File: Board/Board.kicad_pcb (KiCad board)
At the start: 2 copper layers, 71.1 x 58.4 mm, 16 parts, among them J1 Bluetooth, J2 Conn_01x04_Female, J4 Conn_01x03_Female, J5 Conn_01x04_Female, J6 Voltage In 1, J7 Voltage In 2, J8 TrnasistorNPN

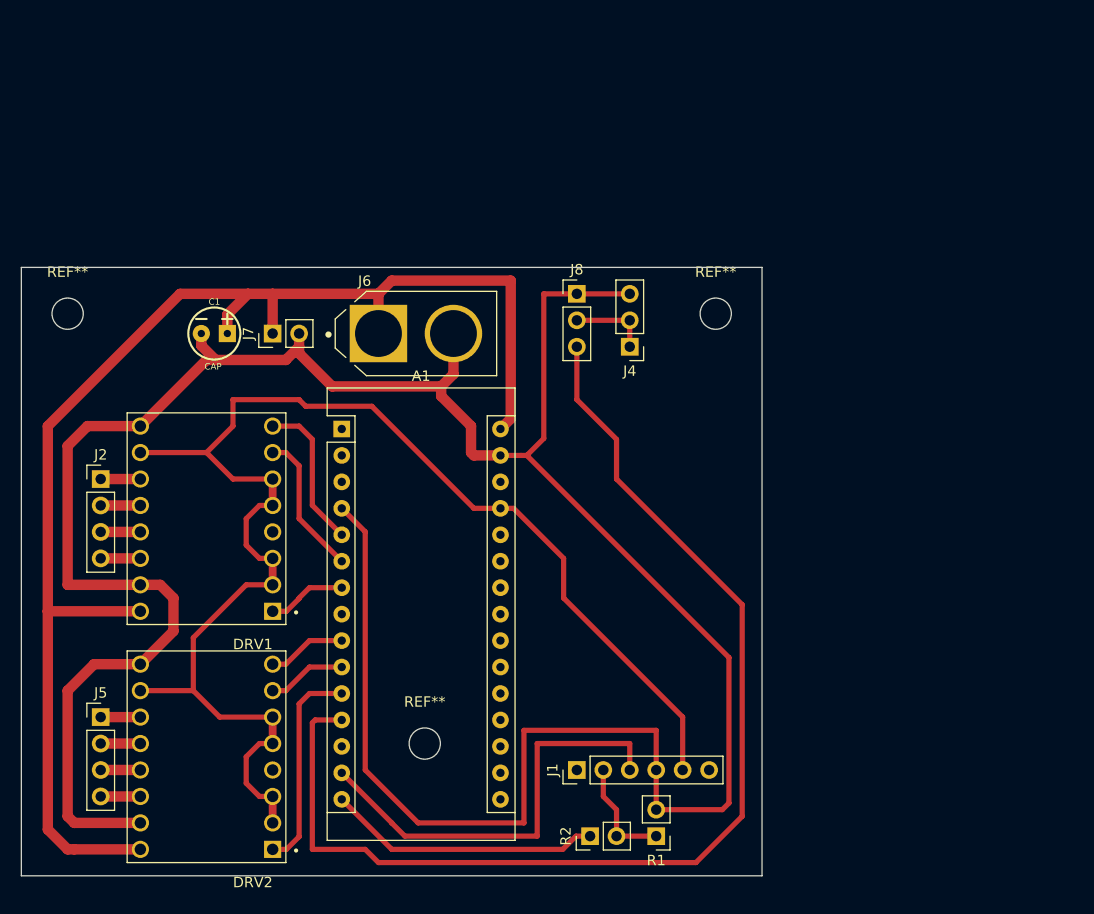
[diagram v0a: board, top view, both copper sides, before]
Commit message: now its perfect
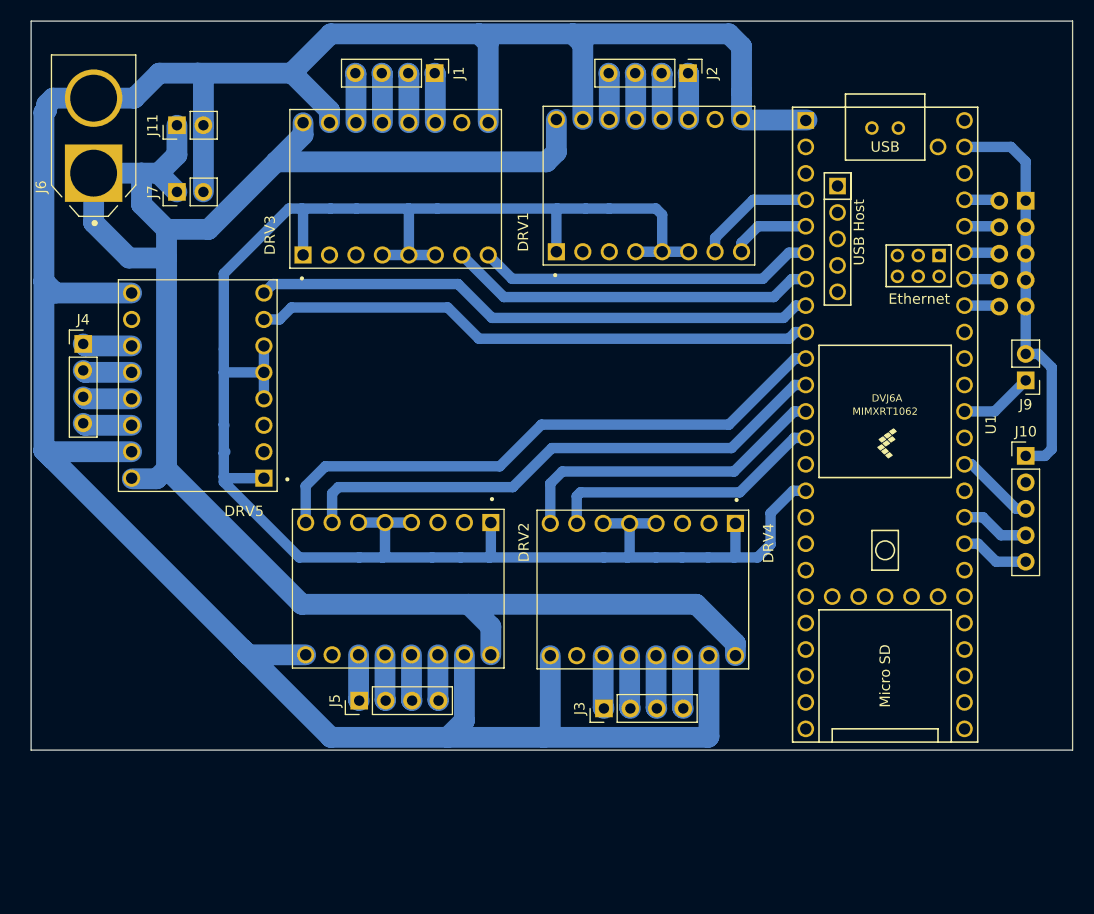
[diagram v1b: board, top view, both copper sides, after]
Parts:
- removed A1: Arduino_Nano_v3.x, Module:Arduino_Nano
- removed C1: CAP, Capacitors:CPOL-RADIAL-2.5MM-5MM
- removed R1: 2K, Connector_PinHeader_2.54mm:PinHeader_1x02_P2.54mm_Vertical
- removed R2: 1K, Connector_PinHeader_2.54mm:PinHeader_1x02_P2.54mm_Vertical
- removed REF** (x3): MountingHole_3mm, MountingHole:MountingHole_3mm
- added DRV3: Y1 Driver, DRV8825_STEPPER_MOTOR_DRIVER_CARRIER:IC_DRV8825_STEPPER_MOTOR_DRIVER_CARRIER, F.Cu at (135.0, -13.9)
- added DRV4: Y2 Driver, DRV8825_STEPPER_MOTOR_DRIVER_CARRIER:IC_DRV8825_STEPPER_MOTOR_DRIVER_CARRIER, F.Cu at (158.7, 24.6)
- added DRV5: Z1 Driver, DRV8825_STEPPER_MOTOR_DRIVER_CARRIER:IC_DRV8825_STEPPER_MOTOR_DRIVER_CARRIER, F.Cu at (116.0, 5.00)
- added J10: Conn_01x05_Female, Connector_PinHeader_2.54mm:PinHeader_1x05_P2.54mm_Vertical, F.Cu at (195.5, 11.8)
- added J11: CAP, Connector_PinHeader_2.54mm:PinHeader_1x02_P2.54mm_Vertical, F.Cu at (114.0, -20.0)
- added J3: Conn_01x04_Female, Connector_PinHeader_2.54mm:PinHeader_1x04_P2.54mm_Vertical, F.Cu at (155.0, 36.0)
- added J9: Probe Header, Connector_PinHeader_2.54mm:PinHeader_1x02_P2.54mm_Vertical, F.Cu at (195.5, 4.50)
- added U1: Teensy4.1, teensy:Teensy41, F.Cu at (182.0, 8.75)
- DRV1: value DRV8825_STEPPER_MOTOR_DRIVER_CARRIER -> X1 Driver
- DRV2: value DRV8825_STEPPER_MOTOR_DRIVER_CARRIER -> X2 Driver
- J1: value Bluetooth -> Conn_01x04_Female; footprint Connector_PinHeader_2.54mm:PinHeader_1x06_P2.54mm_Vertical -> Connector_PinHeader_2.54mm:PinHeader_1x04_P2.54mm_Vertical
- J4: value Conn_01x03_Female -> Conn_01x04_Female; footprint Connector_PinHeader_2.54mm:PinHeader_1x03_P2.54mm_Vertical -> Connector_PinHeader_2.54mm:PinHeader_1x04_P2.54mm_Vertical
- J8: value TrnasistorNPN -> Conn_02x05_Odd_Even; footprint Connector_PinHeader_2.54mm:PinHeader_1x03_P2.54mm_Vertical -> Connector_PinHeader_2.54mm:PinHeader_2x05_P2.54mm_Vertical; moved to B.Cu
- moved J2 68.6 mm to (163.1, -25.0), turned to 270 degrees
- moved J1 68.3 mm to (138.8, -25.0), turned to 270 degrees
- moved DRV1 53.2 mm to (159.3, -14.2), turned to 90 degrees
- moved J4 52.5 mm to (105.0, 1.00), turned to 0 degrees
- moved J8 44.0 mm to (195.5, -12.8), turned to 180 degrees
- moved J6 36.3 mm to (106.0, -19.0), turned to 90 degrees
- moved J5 24.9 mm to (131.5, 35.2), turned to 90 degrees
- moved DRV2 24.5 mm to (135.2, 24.5), turned to 270 degrees
- moved J7 16.4 mm to (114.0, -13.6)
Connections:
- DRV1 pad 1: Net-(A1-Pad7) -> 3V
- DRV1 pad 10: 5V -> Net-(DRV1-Pad10)
- DRV1 pad 2: 5V -> Net-(DRV1-Pad2)
- DRV1 pad 3: 5V -> Net-(DRV1-Pad3)
- DRV1 pad 4: Net-(DRV1-Pad4) -> 3V
- DRV1 pad 5: 5V -> 3V
- DRV1 pad 6: 5V -> 3V
- DRV1 pad 7: Net-(A1-Pad6) -> STEP1
- DRV1 pad 8: Net-(A1-Pad5) -> DIR1
- DRV2 pad 1: Net-(A1-Pad11) -> 3V
- DRV2 pad 10: 5V -> Net-(DRV2-Pad10)
- DRV2 pad 2: 5V -> Net-(DRV2-Pad2)
- DRV2 pad 3: 5V -> Net-(DRV2-Pad3)
- DRV2 pad 4: Net-(DRV2-Pad4) -> 3V
- DRV2 pad 5: 5V -> 3V
- DRV2 pad 6: 5V -> 3V
- DRV2 pad 7: Net-(A1-Pad10) -> STEP2
- DRV2 pad 8: Net-(A1-Pad9) -> DIR2
- J1 pad 4: GND -> Net-(DRV3-Pad14)
- J4 pad 1: DRAIN -> Net-(DRV5-Pad11)
- J4 pad 2: DRAIN -> Net-(DRV5-Pad12)
- J4 pad 3: GND -> Net-(DRV5-Pad13)
- J8 pad 2: DRAIN -> Limit5
- J8 pad 3: Shutter -> GND
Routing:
- net 3V: track 0.00 -> 192.0 mm
- net 5V: track 139.1 -> 0.00 mm
- net Shutter: track 110.4 -> 0.00 mm
- net DIR2: track 0.00 -> 56.6 mm
- net DIR5: track 0.00 -> 54.2 mm
- net STEP5: track 0.00 -> 54.0 mm
- net STEP2: track 0.00 -> 52.6 mm
- net GND: track 269.5 -> 315.3 mm
- net 12V: track 134.5 -> 177.3 mm
- net Net-(DRV3-Pad13): track 41.6 -> 4.78 mm
- net STEP3: track 0.00 -> 35.4 mm
- net DIR3: track 0.00 -> 32.5 mm
- net DIR4: track 0.00 -> 31.2 mm
- net STEP4: track 0.00 -> 26.9 mm
- net Net-(A1-Pad15): track 26.4 -> 0.00 mm
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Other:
- board size 71.1 x 58.4 mm -> 100 x 70 mm
